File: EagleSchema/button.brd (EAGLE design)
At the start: 21.5 x 56 mm, 38 parts, among them IC1 TP4056

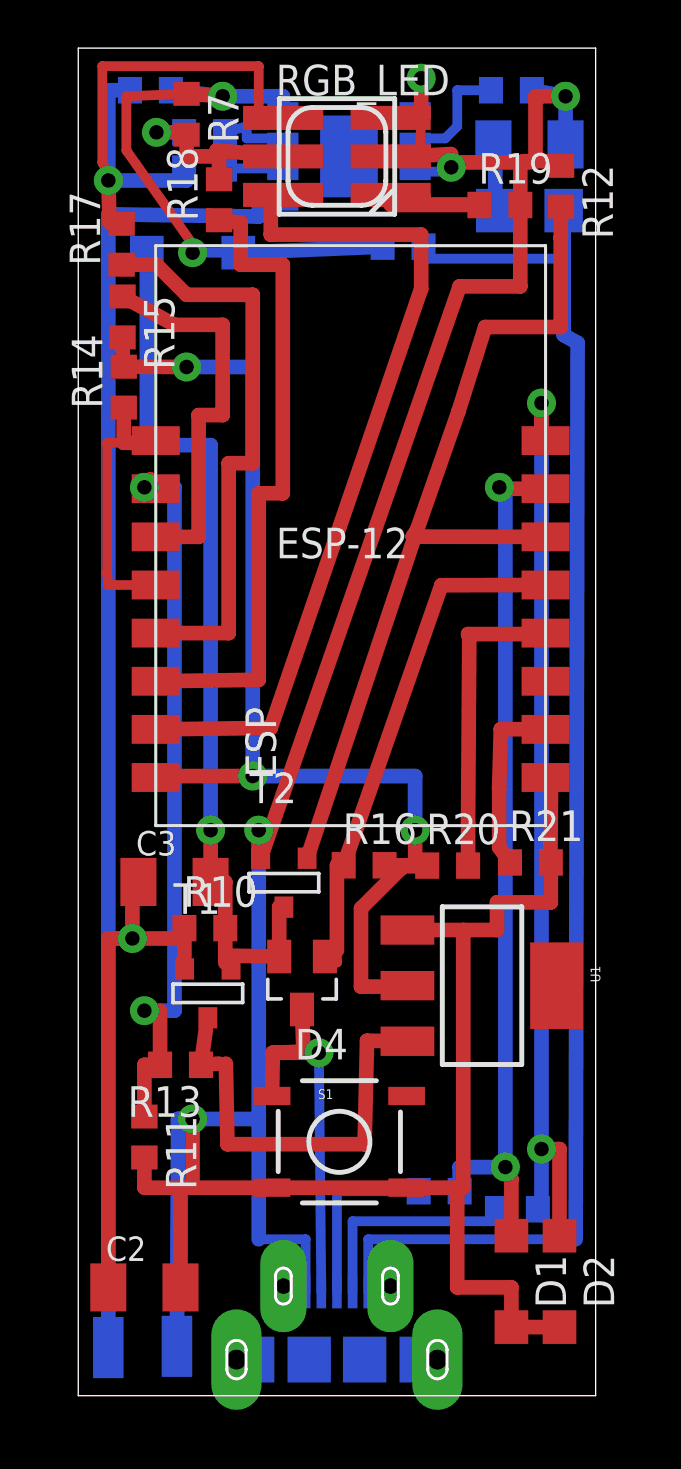
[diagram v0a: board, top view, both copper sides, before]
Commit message: new version
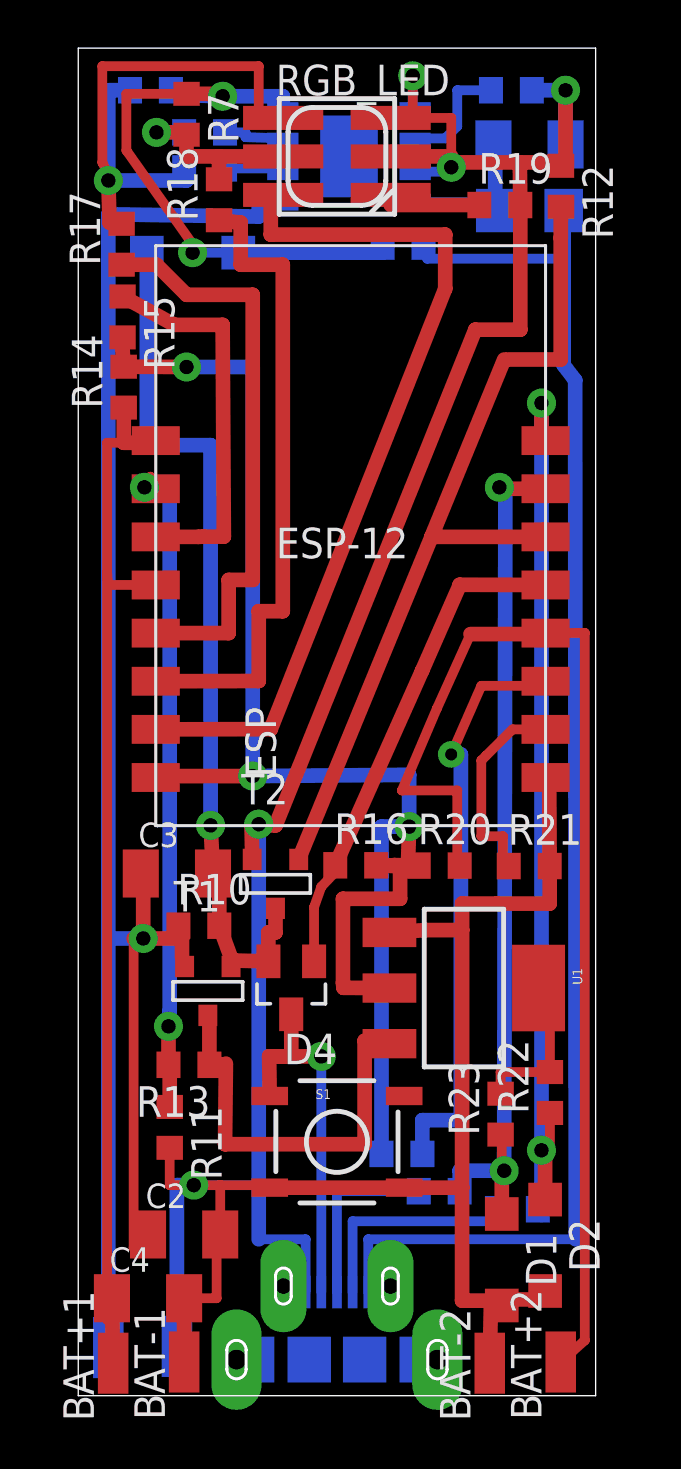
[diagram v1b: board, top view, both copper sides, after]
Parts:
- added BAT+1, BAT+2, BAT-1, BAT-2: WIREPADSMD1,27-254, wirepad:SMD1,27-2,54
- added C4: 0.1, resistor:C1206K
- added R22, R23, R24: 103, resistor:R0603
- moved C2 2.75 mm to (4.40, 6.70)
- moved D2 1.62 mm to (19.4, 6.25)
- moved R11 1.12 mm to (3.80, 11.2)
- moved D1 0.98 mm to (17.6, 5.65)
- moved U1 0.76 mm to (16.0, 16.9)
- moved D4 0.49 mm to (8.85, 16.9)
- moved C3 0.36 mm to (4.10, 21.7)
- moved T2 0.35 mm to (8.17, 21.3)
- moved R16 0.35 mm to (11.5, 22.0)
- moved R13 0.35 mm to (4.60, 13.8)
- moved R20 0.35 mm to (15.0, 22.0)
- moved R10 0.27 mm to (5.01, 19.5)
- moved R21 0.16 mm to (18.7, 22.0)
- moved T1 0.10 mm to (5.36, 16.8)
- moved S1 0.10 mm to (10.8, 10.6)
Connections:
- new net N$17: ESP.11, R24.2
- new net N$29: R22.2, R23.2, U1.4
- net GND: now also BAT-1.1, BAT-2.1, C4.2
- net N$10: now also BAT+2.1
- net N$12: now also R24.1
- net N$27: now also R23.1
- net N$28: now also R22.1
- net N$7: now also BAT+1.1, C4.1
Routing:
- net N$10: track 12.9 -> 48.2 mm
- net N$7: track 11.4 -> 46.1 mm
- net N$17: track 0.00 -> 24.6 mm, vias 0 -> 1
- net N$12: track 50.4 -> 65.9 mm
- net N$29: track 0.00 -> 6.96 mm
- net GND: track 150.3 -> 154.2 mm
- net N$15: track 31.0 -> 27.9 mm
- net N$4: track 78.6 -> 76.8 mm
- net N$8: track 34.8 -> 36.2 mm
- net N$2: track 38.0 -> 36.8 mm
- net N$11: track 7.55 -> 8.64 mm
- net N$30: track 9.34 -> 8.28 mm
- net N$1: track 18.0 -> 17.2 mm
- net N$3: track 21.5 -> 21.0 mm
- net N$27: track 36.2 -> 36.8 mm
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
